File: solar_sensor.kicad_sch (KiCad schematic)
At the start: 3 parts

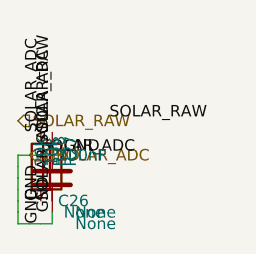
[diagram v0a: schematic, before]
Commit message: fix writer
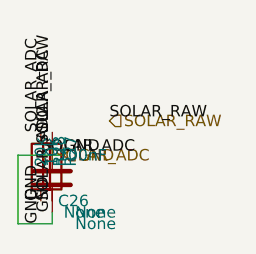
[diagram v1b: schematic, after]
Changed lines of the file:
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@@
 		(instances
 			(project "Untitled"
-				(path "/409c93fd-bba0-4dd0-8760-a3cdb1c560b2"
+				(path "/232a395d-dcd7-4c92-b9dd-1bda61371bf3"
 					(reference "C26")
 					(unit 1)
@@
 		(instances
 			(project "Untitled"
-				(path "/409c93fd-bba0-4dd0-8760-a3cdb1c560b2"
+				(path "/232a395d-dcd7-4c92-b9dd-1bda61371bf3"
 					(reference "R27")
 					(unit 1)
@@
 		(instances
 			(project "Untitled"
-				(path "/409c93fd-bba0-4dd0-8760-a3cdb1c560b2"
+				(path "/232a395d-dcd7-4c92-b9dd-1bda61371bf3"
 					(reference "R28")
 					(unit 1)
@@
 	(wire
 		(pts
-			(xy 17.78 24.13) (xy 16.51 24.13)
-		)
-		(stroke
-			(width 0)
-			(type default)
-		)
-	)
-	(wire
-		(pts
-			(xy 16.51 24.13) (xy 15.24 24.13)
-		)
-		(stroke
-			(width 0)
-			(type default)
-		)
-	)
-	(wire
-		(pts
-			(xy 15.24 24.13) (xy 13.97 24.13)
-		)
-		(stroke
-			(width 0)
-			(type default)
-		)
-	)
-	(wire
-		(pts
-			(xy 13.97 24.13) (xy 13.97 22.86)
-		)
-		(stroke
-			(width 0)
-			(type default)
-		)
-	)
-	(wire
-		(pts
-			(xy 13.97 22.86) (xy 13.97 21.59)
-		)
-		(stroke
-			(width 0)
-			(type default)
-		)
-	)
-	(wire
-		(pts
-			(xy 13.97 21.59) (xy 13.97 20.32)
-		)
-		(stroke
-			(width 0)
-			(type default)
-		)
-	)
-	(wire
-		(pts
-			(xy 13.97 20.32) (xy 13.97 19.05)
-		)
-		(stroke
-			(width 0)
-			(type default)
-		)
-	)
-	(wire
-		(pts
-			(xy 13.97 19.05) (xy 13.97 17.78)
-		)
-		(stroke
-			(width 0)
-			(type default)
-		)
-	)
-	(wire
-		(pts
-			(xy 13.97 17.78) (xy 13.97 16.51)
+			(xy 17.78 24.13) (xy 13.97 24.13)
+		)
+		(stroke
+			(width 0)
+			(type default)
+		)
+	)
+	(wire
+		(pts
+			(xy 13.97 24.13) (xy 13.97 16.51)
 		)
 		(stroke
@@
 	(hierarchical_label "GND"
 		(shape input)
-		(at 15.24 16.51 180)
+		(at 19.05 16.51 180)
 		(effects
 			(font
@@
 	(hierarchical_label "SOLAR_RAW"
 		(shape input)
-		(at 13.97 12.7 180)
-		(effects
-			(font
+		(at 24.13 12.7 180)
+		(effects
+			(font
